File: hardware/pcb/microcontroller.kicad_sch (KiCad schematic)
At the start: 46 parts, among them J3 TYPE-C sinking plate, Q1 2N7002VC-, Q2 2N7002VC-, SW18 SWITCH, U1 W25Q64JV, U3 USBLC6-2P6, U4 XC6206P332MR-G, U6 RP2040, U7 74LVC1T45, Y1 12MHz

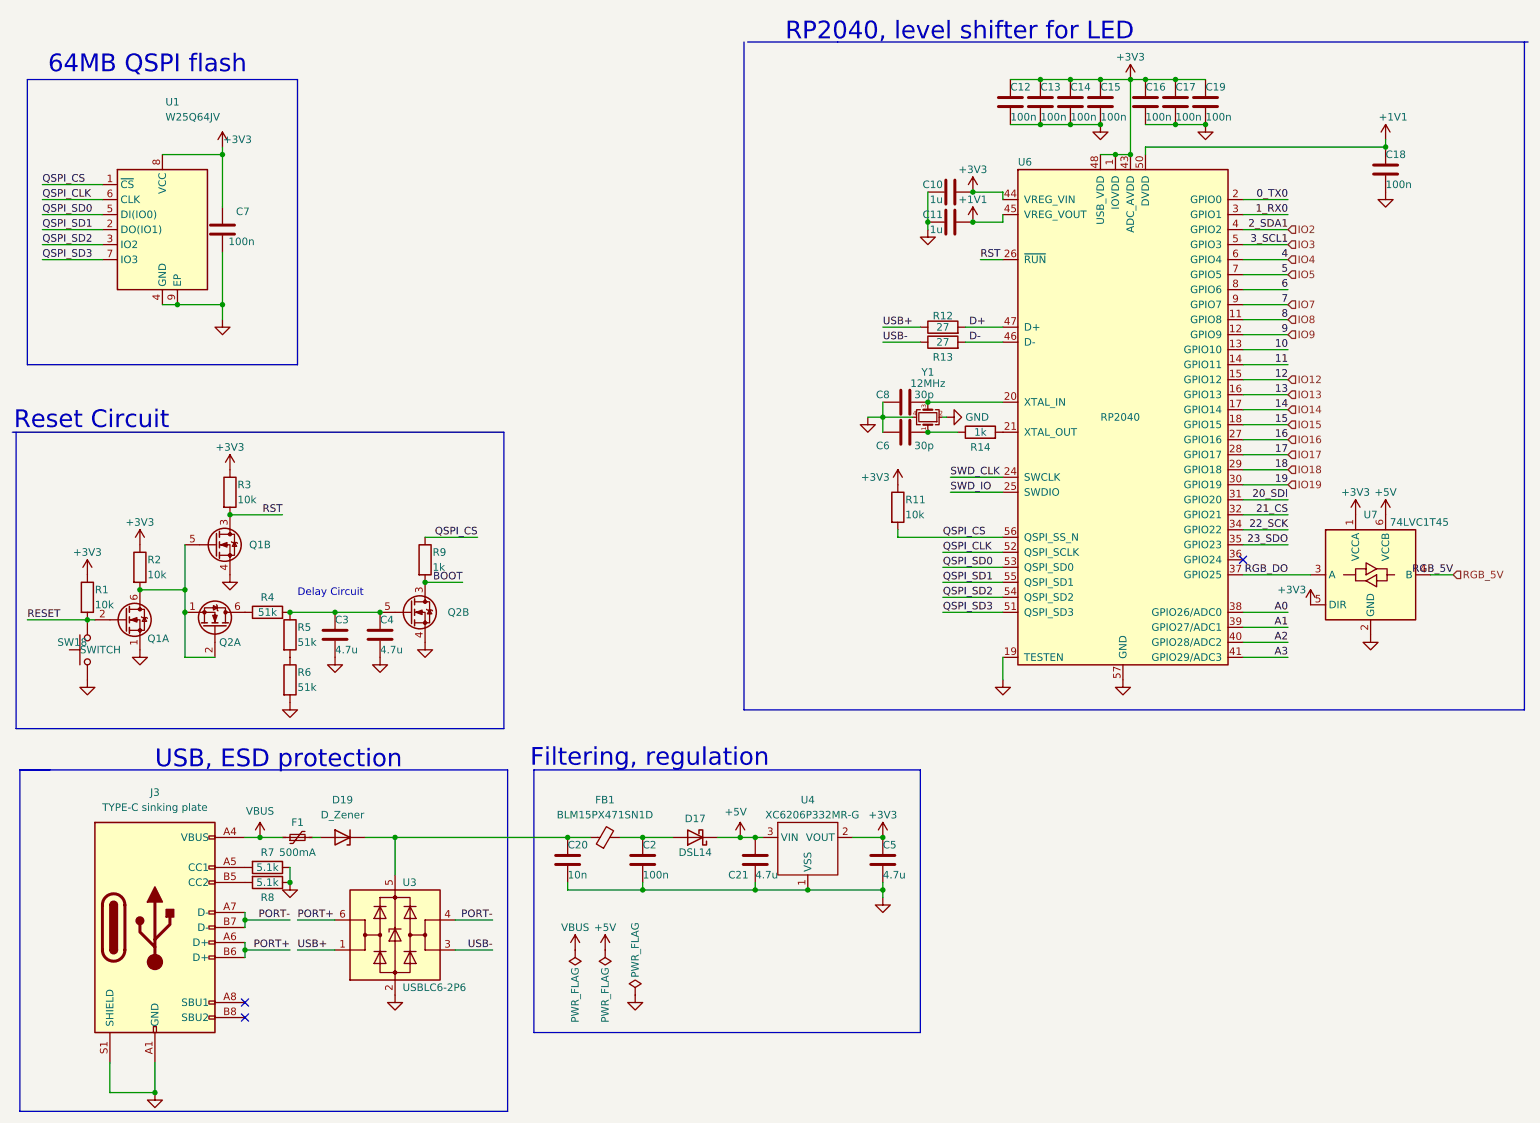
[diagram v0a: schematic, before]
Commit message: Version 1.5
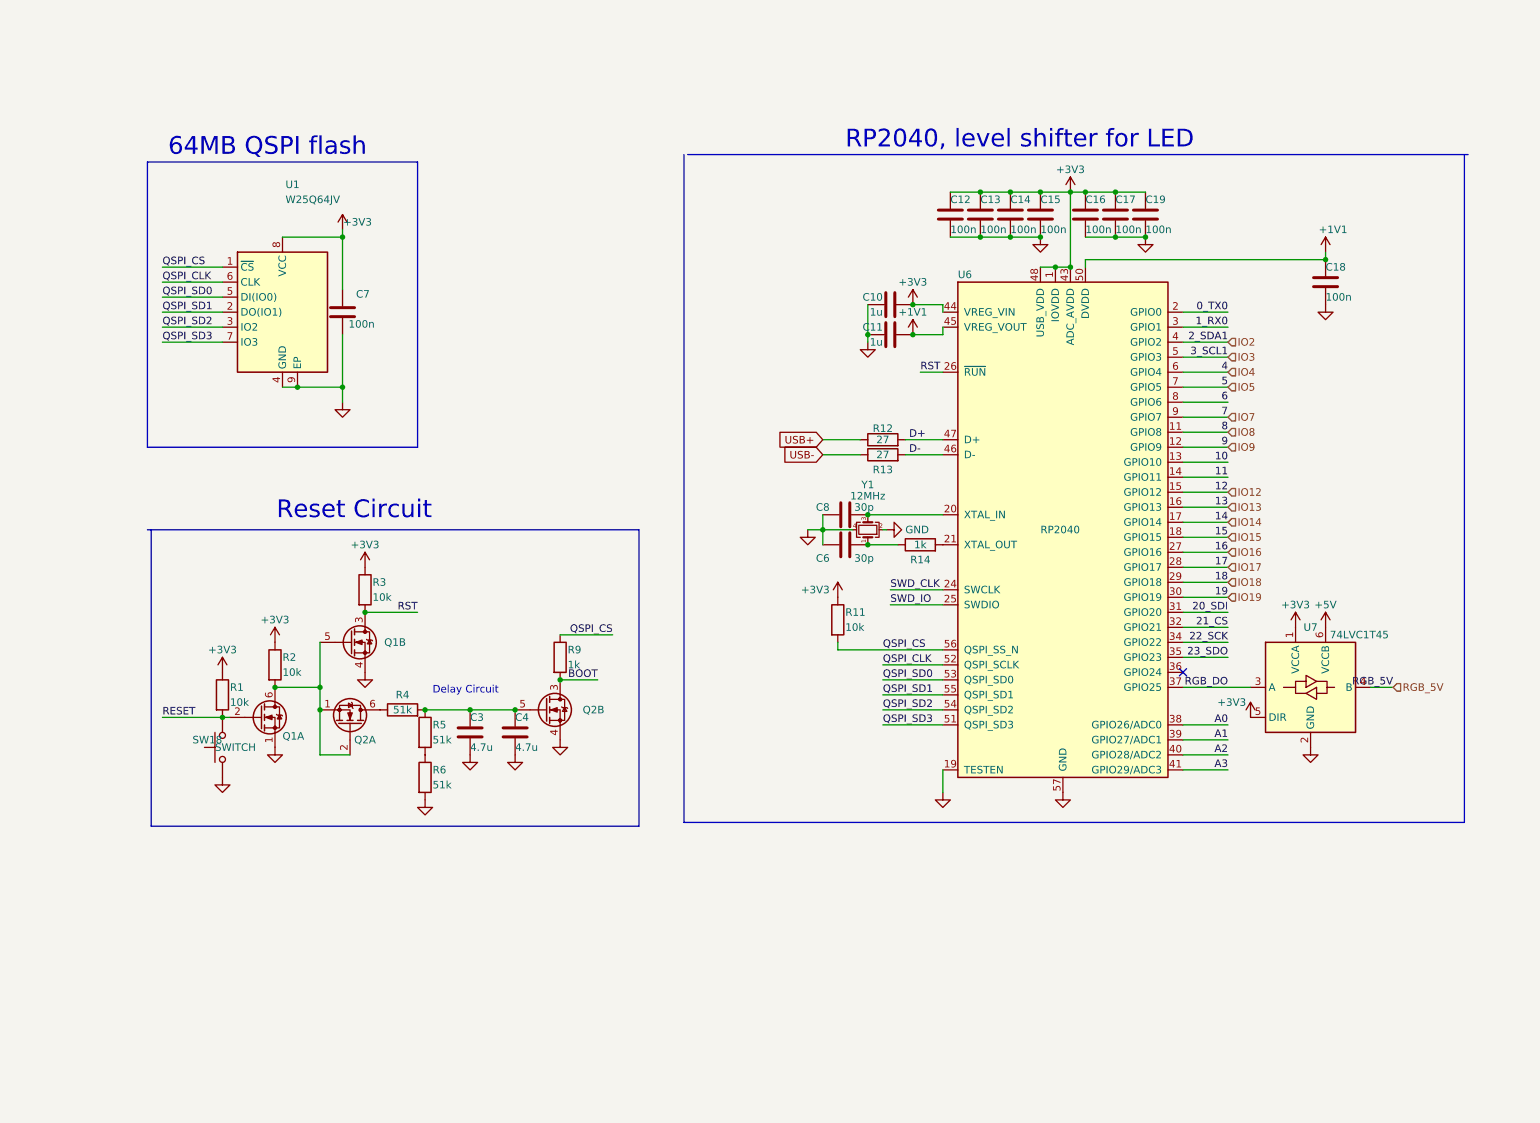
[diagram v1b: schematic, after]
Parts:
- removed C2: 100n, Capacitor_SMD:C_0402_1005Metric, symbol Device:C
- removed C20: 10n, Capacitor_SMD:C_0603_1608Metric, symbol Device:C
- removed C21, C5: 4.7u, Capacitor_SMD:C_0402_1005Metric, symbol Device:C
- removed D17: DSL14, Diode_SMD:D_SOD-123, symbol Device:D_Schottky
- removed D19: D_Zener, mathboard:DFN1006-2L, symbol Device:D_Zener
- removed F1: 500mA, Fuse:Fuse_0402_1005Metric, symbol Device:Polyfuse_Small
- removed FB1: BLM15PX471SN1D, Inductor_SMD:L_0402_1005Metric, symbol Device:FerriteBead_Small
- removed J3: TYPE-C sinking plate, mathboard:USB_C_Receptacle_XYECONN TYPE-C-F02C-1BBWC1.6, symbol Connector:USB_C_Receptacle_USB2.0
- removed R7, R8: 5.1k, Resistor_SMD:R_0402_1005Metric, symbol Device:R
- removed U3: USBLC6-2P6, Package_TO_SOT_SMD:SOT-666, symbol Power_Protection:USBLC6-2P6
- removed U4: XC6206P332MR-G, Package_TO_SOT_SMD:SOT-23, symbol Mathboard:XC6206P332MR-G
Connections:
- no-connect marks 3 -> 1
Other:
- note removed: "Filtering, regulation"
- note removed: "USB, ESD protection"
- moved on the sheet: C10, C11, C12, C13, C14, C15, C16, C17, C18, C19, C3, C4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
